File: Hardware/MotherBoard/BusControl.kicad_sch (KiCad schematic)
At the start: 3 parts, among them U6 74HC20, U7 74HC10, U8 74HC04

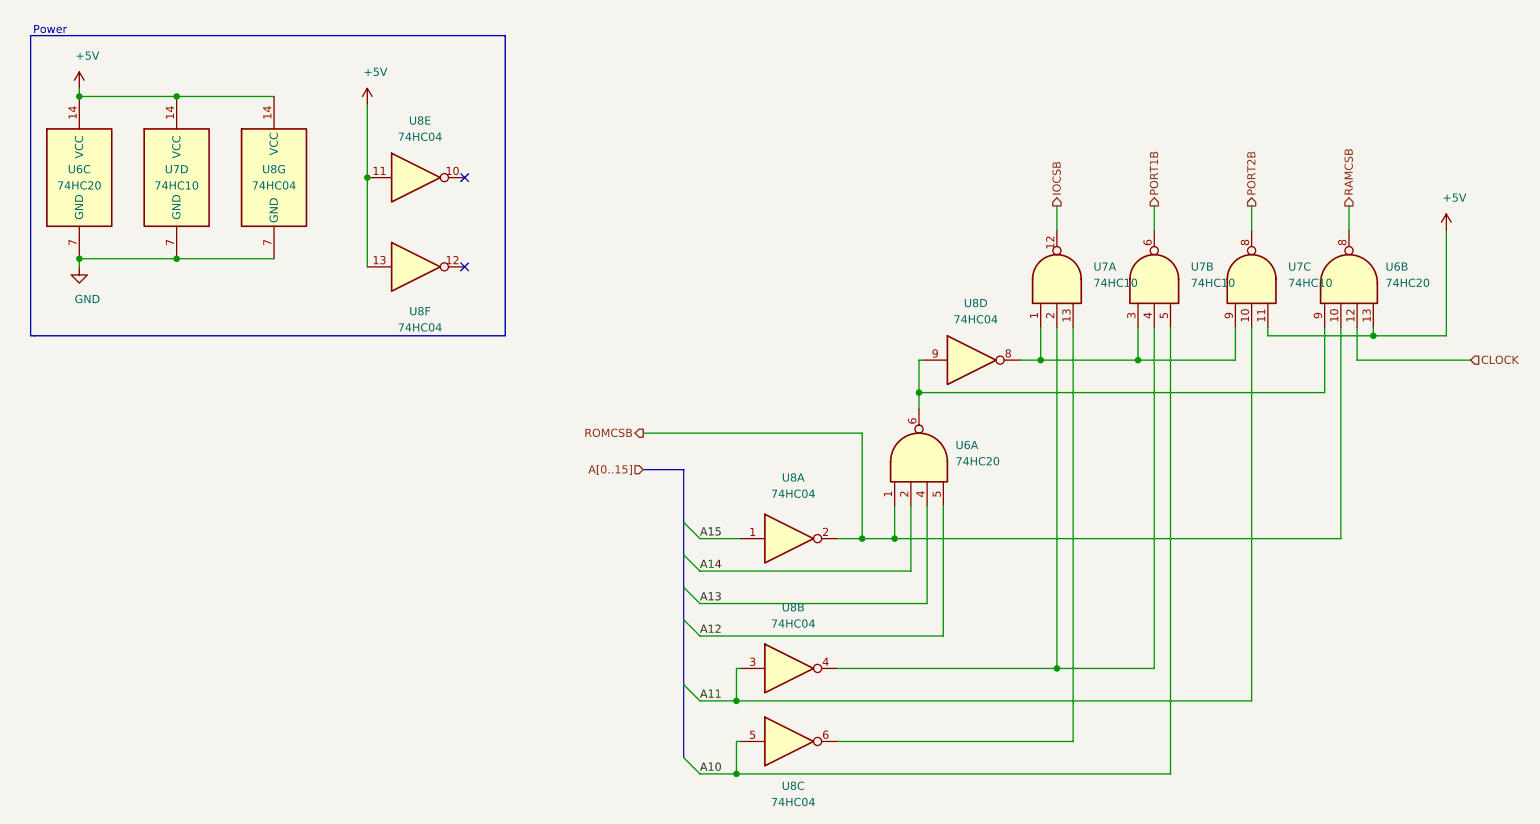
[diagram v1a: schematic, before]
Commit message: Version 1.2
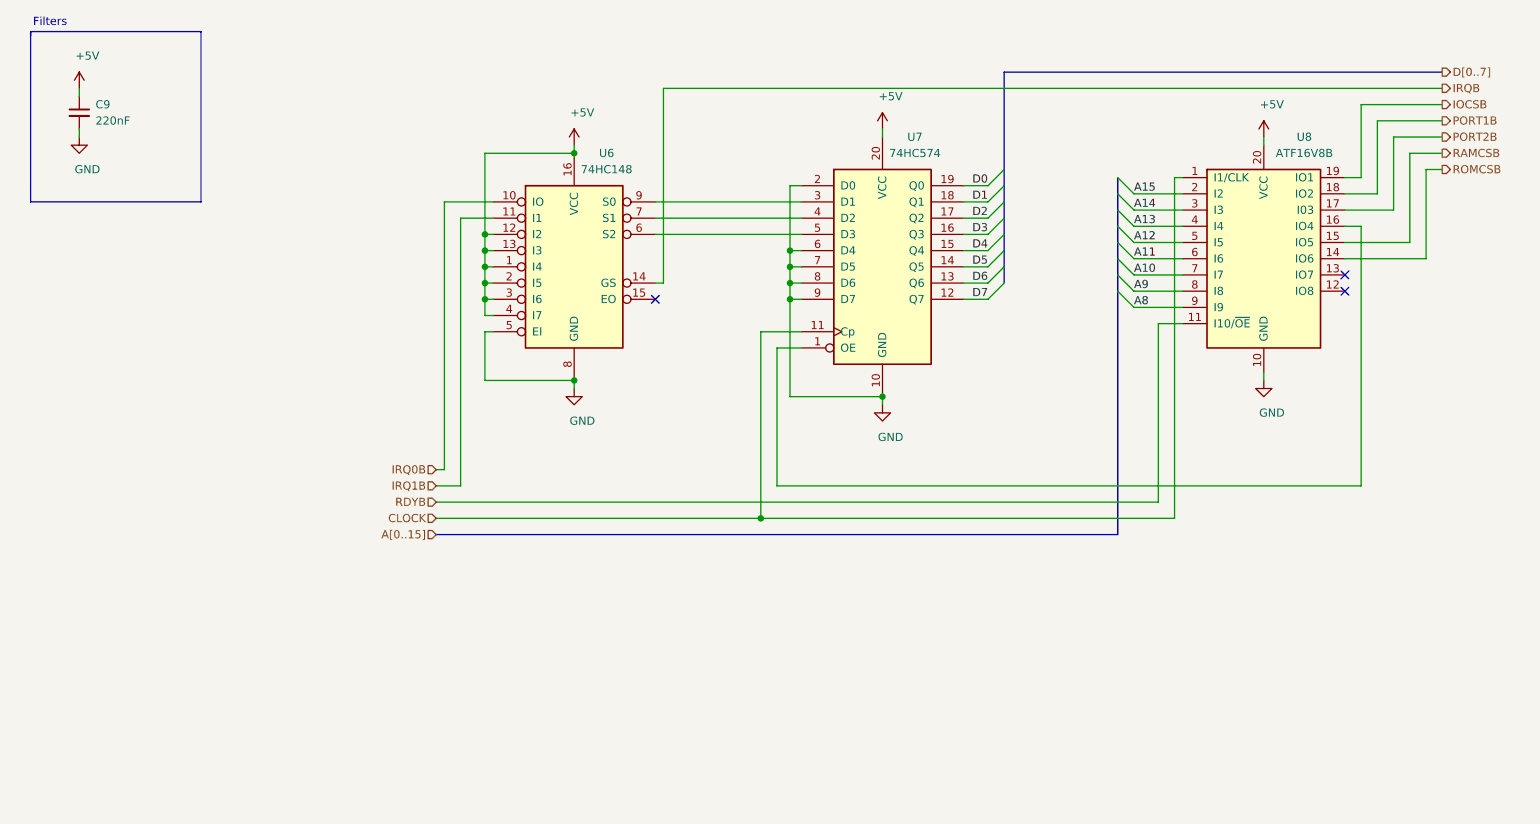
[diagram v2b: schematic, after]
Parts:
- removed U6: 74HC20, Package_DIP:DIP-14_W7.62mm, symbol 74xx:74LS20
- removed U7: 74HC10, Package_DIP:DIP-14_W7.62mm, symbol 74xx:74LS10
- removed U8: 74HC04, Package_DIP:DIP-14_W7.62mm, symbol 74xx:74LS04
- added C9: 220nF, Capacitor_THT:C_Disc_D5.0mm_W2.5mm_P5.00mm, symbol Device:C_Small
- added U6: 74HC148, Package_DIP:DIP-16_W7.62mm, symbol 74xx:74LS148
- added U7: 74HC574, Package_DIP:DIP-20_W7.62mm, symbol 74xx:74HCT574
- added U8: ATF16V8B, Package_DIP:DIP-20_W7.62mm, symbol Logic_Programmable:GAL16V8
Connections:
- net +5V: now also C9.1, U6.1 (I4), U6.12 (I2), U6.13 (I3), U6.16 (VCC), U6.2 (I5), U6.3 (I6), U6.4 (I7), U7.20 (VCC), U8.20 (VCC)
- net A10: now also U8.7 (I7)
- net A11: now also U8.6 (I6)
- net A12: now also U8.5 (I5)
- net A13: now also U8.4 (I4)
- net A14: now also U8.3 (I3)
- net A15: now also U8.2 (I2)
- net CLOCK: now also U7.11 (Cp), U8.1 (I1/CLK)
- net GND: now also C9.2, U6.5 (EI), U6.8 (GND), U7.10 (GND), U7.2 (D0), U7.6 (D4), U7.7 (D5), U7.8 (D6), U7.9 (D7), U8.10 (GND)
- net IOCSB: now also U8.19 (IO1)
- net PORT1B: now also U8.18 (IO2)
- net PORT2B: now also U8.17 (I03)
- net RAMCSB: now also U8.15 (IO5)
- net ROMCSB: now also U8.14 (IO6)
- new net: U6.6 (S2), U7.5 (D3)
- new net: U6.7 (S1), U7.4 (D2)
- new net: U6.9 (S0), U7.3 (D1)
- new net: U7.1 (OE), U8.16 (IO4)
- new net A8: U8.9 (I9)
- new net A9: U8.8 (I8)
- new net D0: U7.19 (Q0)
- new net D1: U7.18 (Q1)
- new net D2: U7.17 (Q2)
- new net D3: U7.16 (Q3)
- new net D4: U7.15 (Q4)
- new net D5: U7.14 (Q5)
- new net D6: U7.13 (Q6)
- new net D7: U7.12 (Q7)
- new net IRQ0B: U6.10 (IO)
- new net IRQ1B: U6.11 (I1)
- new net IRQB: U6.14 (GS)
- new net RDYB: U8.11 (I10/~OE~)
- no-connect marks 2 -> 3
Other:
- note added: "Filters"
- note removed: "Power"
